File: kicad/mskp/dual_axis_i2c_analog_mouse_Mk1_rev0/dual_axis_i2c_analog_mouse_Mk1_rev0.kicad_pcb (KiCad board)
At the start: 2 copper layers, 21 parts, among them J1 I2C_controller_JST, J2 I2C_controller_pads, J3 mouse_input_pads, J4 mouse_input_JST, J5 Alert_pad, U1 AMS1117-3.3, U2 ADS1115IDGS

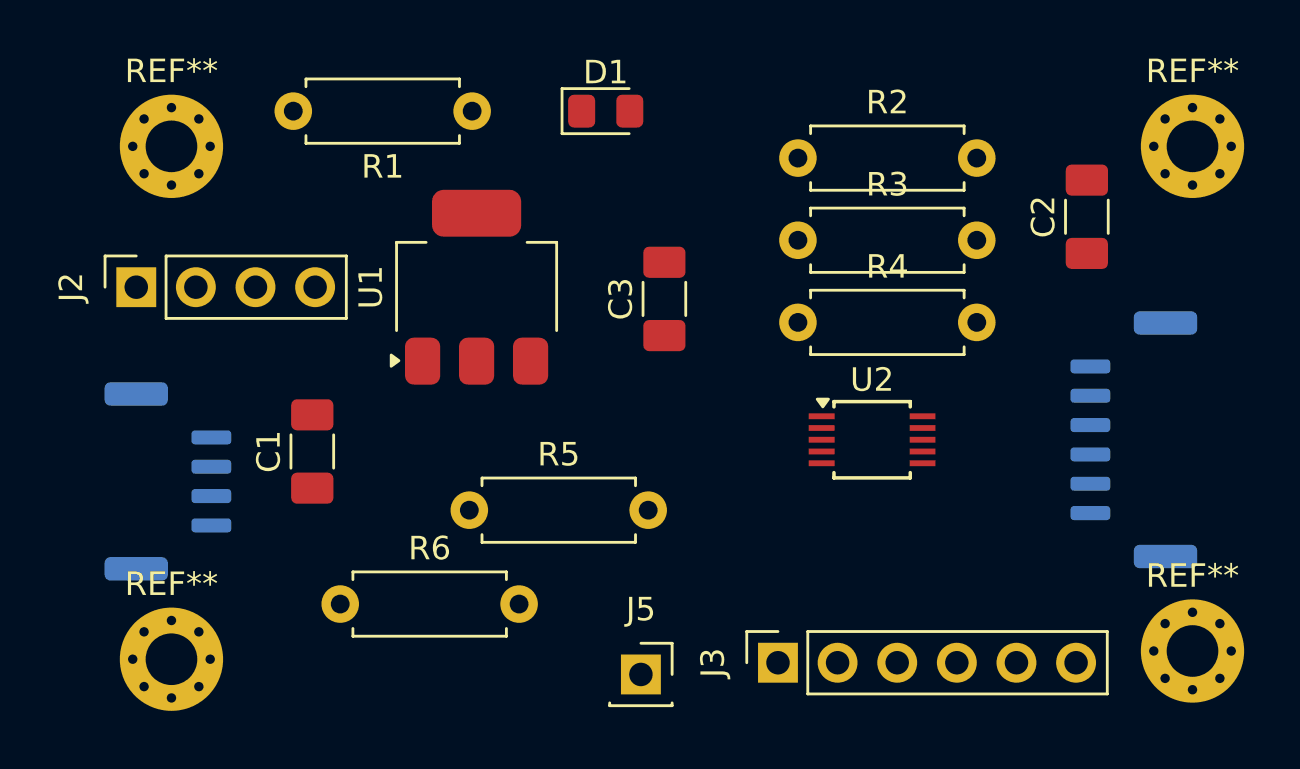
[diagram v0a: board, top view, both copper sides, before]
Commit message: Continues work with rough PCB outlines
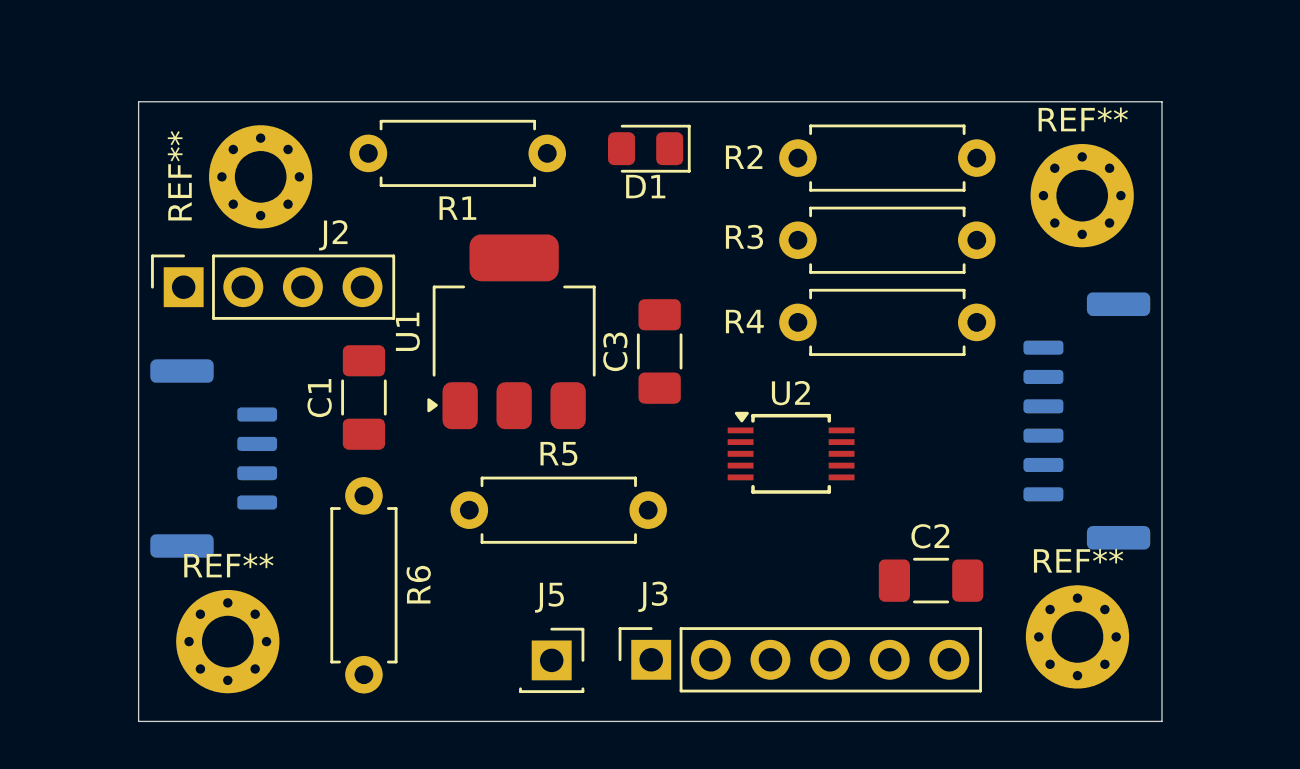
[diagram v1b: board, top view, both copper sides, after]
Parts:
- moved C2 16.9 mm to (138.4, 88.0), turned to 0 degrees
- moved J3 5.40 mm to (126.4, 91.4)
- moved REF** 5.15 mm to (144.8, 71.6)
- moved REF** 4.94 mm to (144.6, 90.4)
- moved R6 4.72 mm to (114.2, 84.4), turned to -90 degrees
- moved REF** 4.02 mm to (109.8, 70.8)
- moved J5 3.85 mm to (122.2, 91.4)
- moved R1 3.67 mm to (122.0, 69.8)
- moved U2 3.50 mm to (132.4, 82.6)
- moved C1 3.18 mm to (114.2, 80.2)
- moved REF** 2.51 mm to (108.4, 90.6)
- moved U1 2.48 mm to (120.6, 77.4)
- moved D1 2.33 mm to (126.2, 69.6), turned to 180 degrees
- moved C3 2.25 mm to (126.8, 78.2)
- moved J1 2.18 mm to (107.8, 82.8)
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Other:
- board outline added: 43.6 x 26.4 mm
